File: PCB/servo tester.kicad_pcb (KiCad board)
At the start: 2 copper layers, 75 x 65 mm, 13 parts, among them SW2 SW_Push, U1 ER_OLEDM0.91_1x-I2C

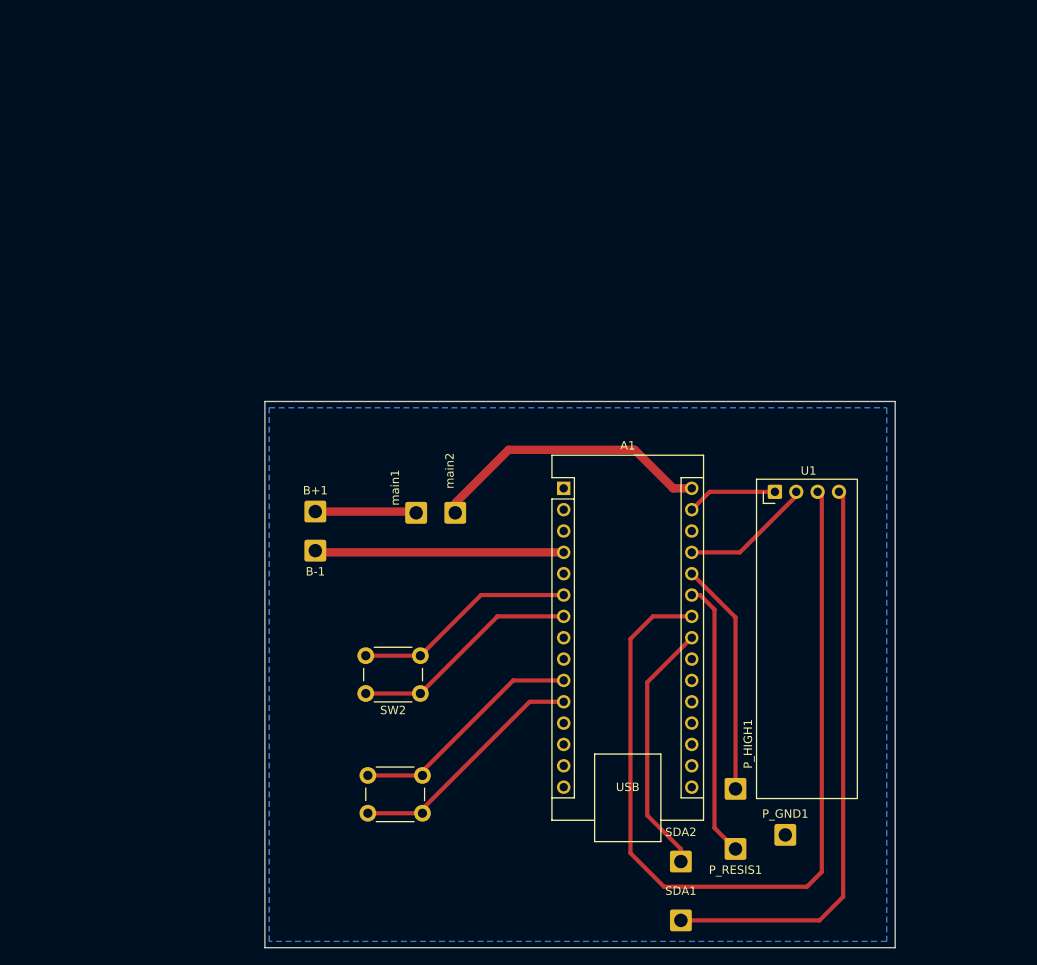
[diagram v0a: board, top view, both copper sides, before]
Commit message: redid pcb
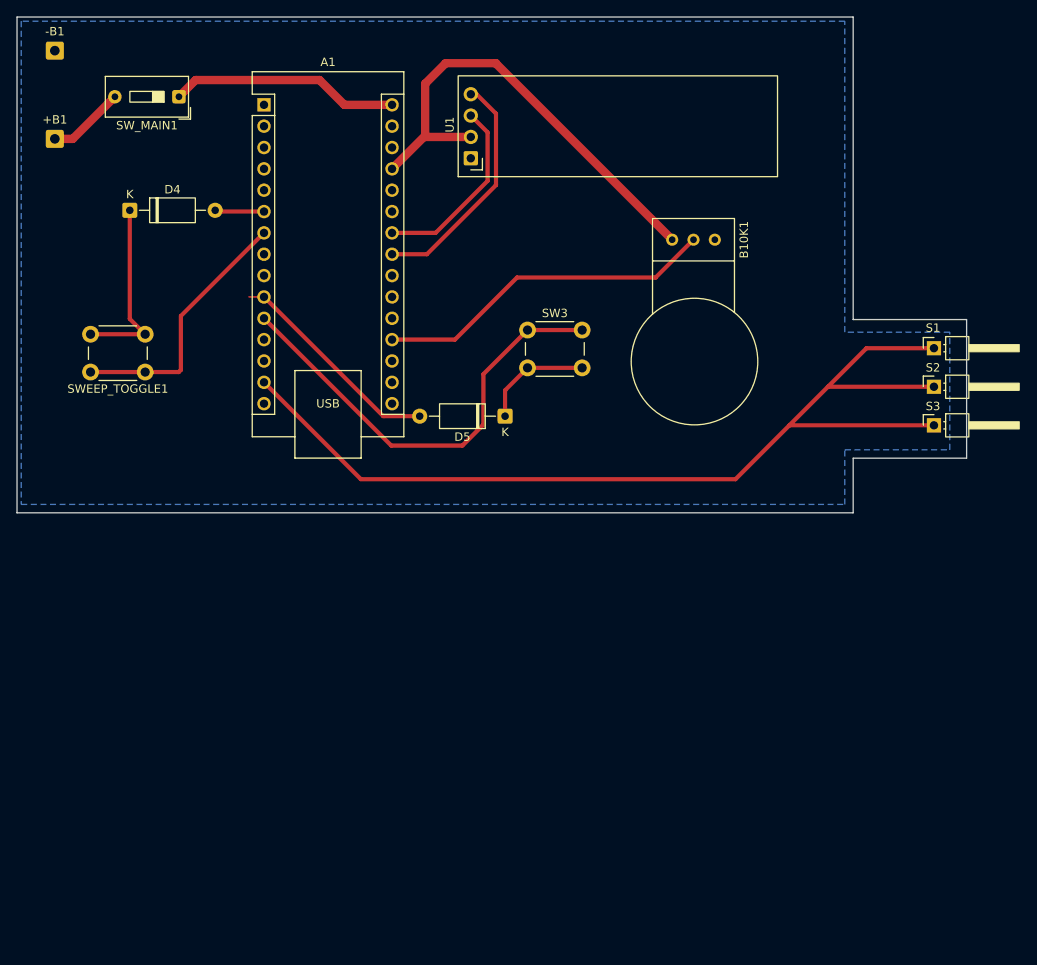
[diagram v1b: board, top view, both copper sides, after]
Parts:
- removed B+1, B-1, P_GND1, P_HIGH1, P_RESIS1, SDA1, SDA2, main1, main2: TestPoint, Connector_Wire:SolderWire-0.75sqmm_1x01_D1.25mm_OD2.3mm
- removed SW2, SWEEPMODE1: SW_Push, Button_Switch_THT:SW_PUSH_6mm_H4.3mm
- added +B1: TestPoint, Connector_Wire:SolderWire-0.5sqmm_1x01_D0.9mm_OD2.1mm, F.Cu at (17.0, 27.0)
- added -B1: TestPoint, Connector_Wire:SolderWire-0.5sqmm_1x01_D0.9mm_OD2.1mm, F.Cu at (17.0, 16.5)
- added B10K1: R_Potentiometer, Potentiometer_THT:Potentiometer_Bourns_3386C_Horizontal, F.Cu at (95.5, 39.0)
- added D4: D, Diode_THT:D_A-405_P10.16mm_Horizontal, F.Cu at (25.9, 35.5)
- added D5: D, Diode_THT:D_A-405_P10.16mm_Horizontal, F.Cu at (70.6, 60.0)
- added S1: Conn_01x01_Pin, Connector_PinHeader_2.54mm:PinHeader_1x01_P2.54mm_Horizontal, F.Cu at (121.6, 51.9)
- added S2: Conn_01x01_Pin, Connector_PinHeader_2.54mm:PinHeader_1x01_P2.54mm_Horizontal, F.Cu at (121.6, 56.5)
- added S3: Conn_01x01_Pin, Connector_PinHeader_2.54mm:PinHeader_1x01_P2.54mm_Horizontal, F.Cu at (121.6, 61.1)
- added SW3: SW_Push, Button_Switch_THT:SW_PUSH_6mm, F.Cu at (73.2, 49.8)
- added SWEEP_TOGGLE1: SW_Push, Button_Switch_THT:SW_PUSH_6mm, F.Cu at (27.8, 54.8)
- added SW_MAIN1: SW_Push, Button_Switch_THT:SW_DIP_SPSTx01_Slide_9.78x4.72mm_W7.62mm_P2.54mm, F.Cu at (31.8, 22.0)
- moved A1 57.9 mm to (41.9, 22.9)
- moved U1 53.7 mm to (66.5, 29.3), turned to 90 degrees
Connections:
- A1 pad 14: unconnected-(A1-D11-Pad14) -> Net-(A1-D11)
- A1 pad 19: unconnected-(A1-A0-Pad19) -> Net-(A1-A0)
- A1 pad 25: Net-(A1-A6) -> unconnected-(A1-A6-Pad25)
- A1 pad 26: Net-(A1-A7) -> unconnected-(A1-A7-Pad26)
- U1 pad 4: Net-(U1-SDA) -> Net-(A1-A4)
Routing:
- net Net-(A1-D11): track 0.00 -> 120.8 mm
- net Net-(A1-A5): track 104.3 -> 22.5 mm
- net Net-(U1-SDA): track 68.7 -> 0.00 mm
- net GND: track 40.9 -> 0.00 mm
- net Net-(A1-A0): track 0.00 -> 40.8 mm
- net Net-(A1-+5V): track 15.9 -> 56.5 mm
- net Net-(A1-A6): track 33.0 -> 0.00 mm
- net Net-(A1-A7): track 27.8 -> 0.00 mm
- net Net-(A1-D8): track 28.6 -> 53.3 mm
- net Net-(D4-K): track 0.00 -> 22.0 mm
- net Net-(A1-D3): track 26.5 -> 5.87 mm
- net Net-(D5-K): track 0.00 -> 13.4 mm
- net Net-(B+1-Pad1): track 12.1 -> 0.00 mm
- net Net-(+B1-Pad1): track 0.00 -> 10.4 mm
- net Net-(A1-VIN): track 33.8 -> 27.4 mm
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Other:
- board size 75 x 65 mm -> 113 x 59 mm
